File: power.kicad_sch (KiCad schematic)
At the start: 108 parts, among them U41 TPS7A8801RTJR, U42 TPS7A8801RTJR, U43 TPS61252DSG, U44 TPSM863252RDXR, U45 TPS7A3301RGW, U46 TPSM863252RDXR

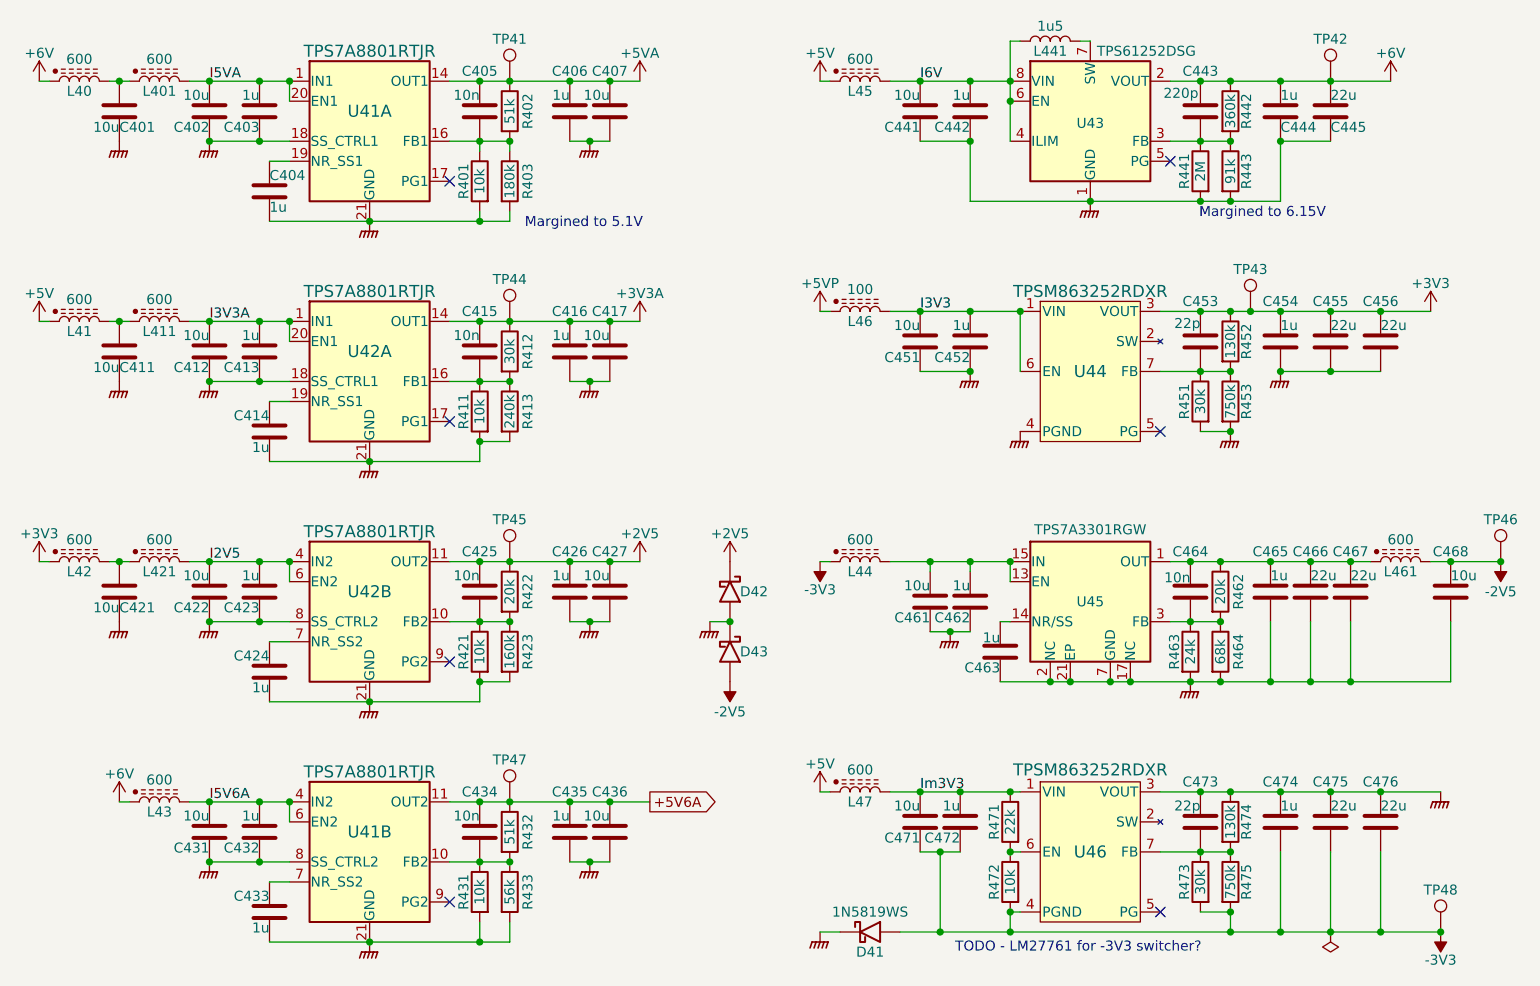
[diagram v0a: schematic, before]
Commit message: Most blocks there....
About to restore scan.
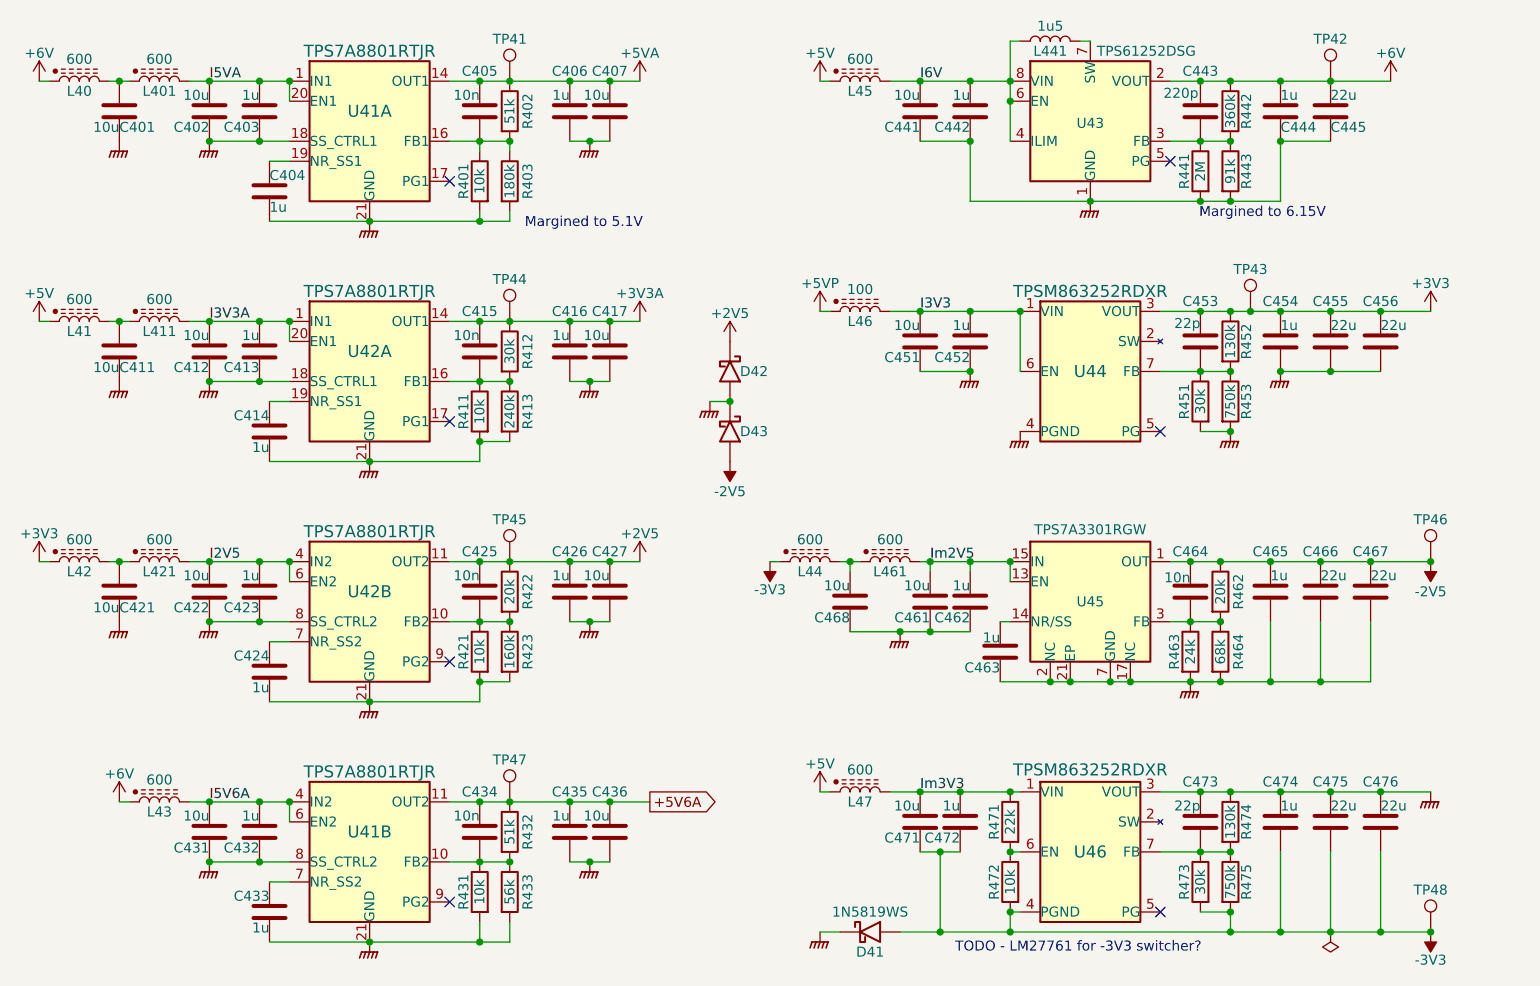
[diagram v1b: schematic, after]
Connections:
- net -2V5: now also C464.1, C465.2, C466.1, C467.1, R462.1, U45.1 (OUT), U45.20 (OUT); no longer C468.1, L461.2
- net Im2V5: now reaches C461.1, C462.1, U45.13 (EN), U45.15 (IN), U45.16 (IN)
- net Im2V5: now also L461.2; no longer L44.2
- new net: C468.1, L44.2, L461.1
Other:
- moved on the sheet: C466, C467, C468, D42, D43, L44, L461, TP46, TP48
